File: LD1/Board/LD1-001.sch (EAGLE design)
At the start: 13 parts, among them IC1 TLC5941NT, IC2 TLC5941NT, IC3 TLC5941NT

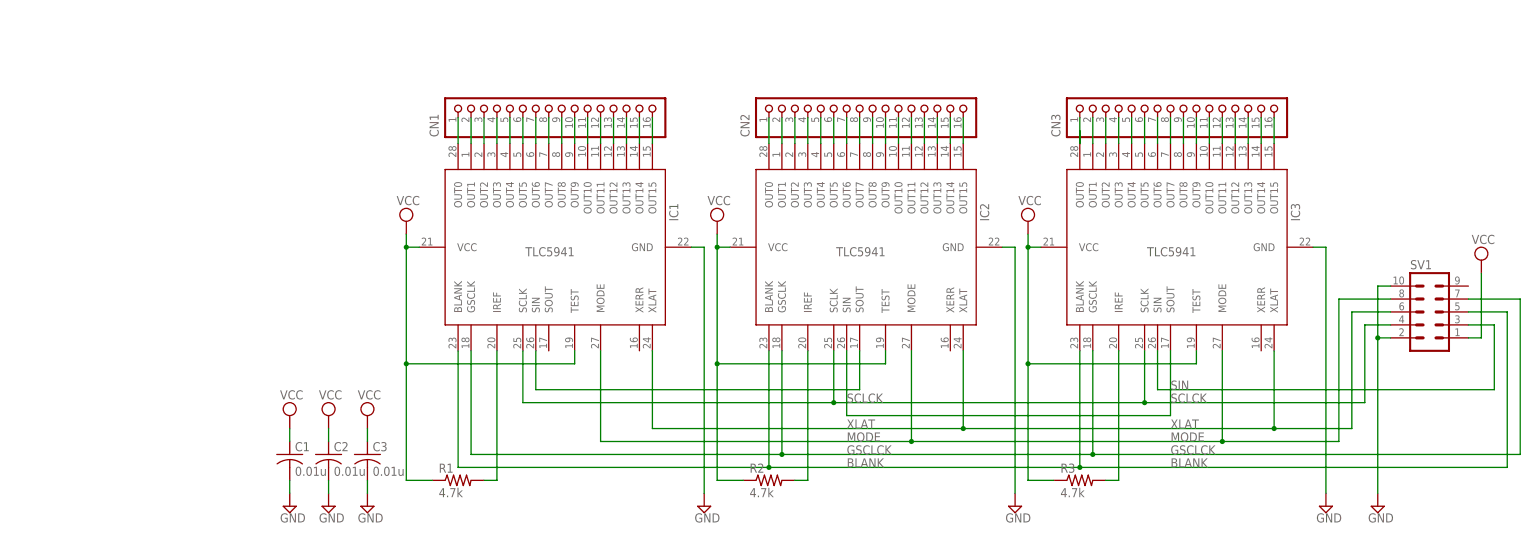
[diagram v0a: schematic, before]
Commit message: Before the first prototyping.
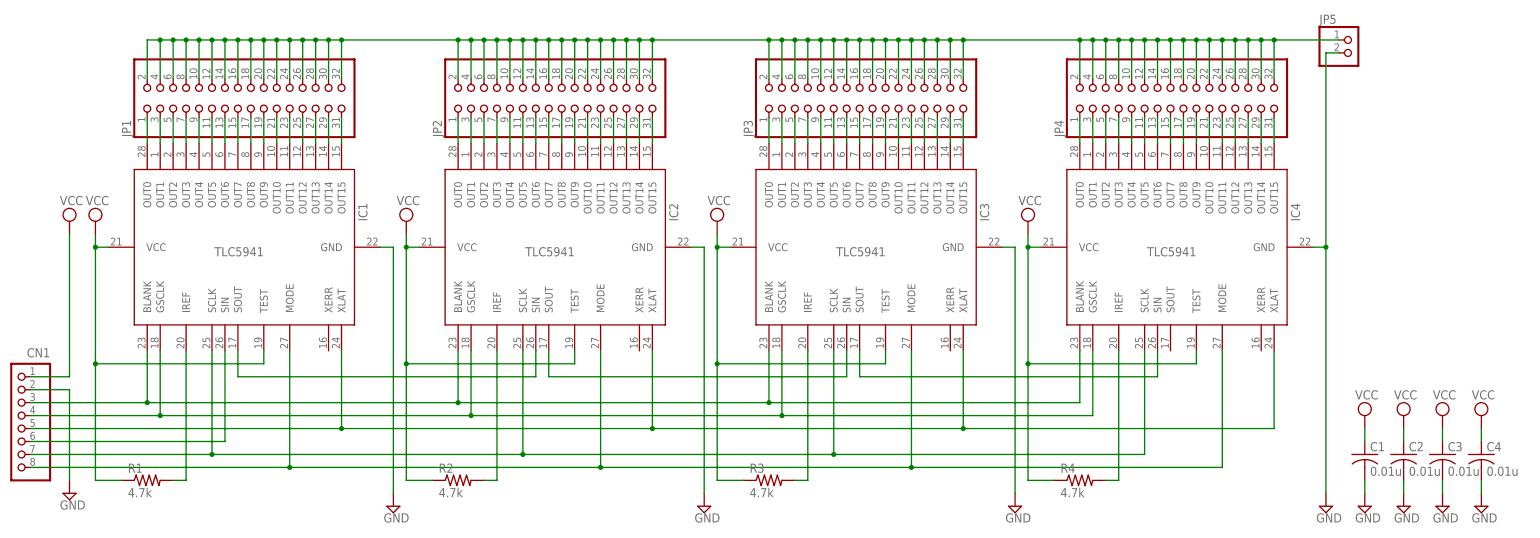
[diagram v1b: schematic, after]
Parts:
- removed CN2, CN3: (no value), jst-ph:B16B-PH-K-S
- removed SV1: (no value), con-ml:ML10
- added C4: 0.01u, rcl:C-US025-025X050
- added IC4: TLC5941NT, adafruit:TLC5941NT
- added JP1, JP2, JP3, JP4: (no value), pinhead:PINHD-2X16
- added JP5: (no value), pinhead:PINHD-1X2
- added R4: 4.7k, resistor:R-US_0204/5
- CN1: device jst-ph:B16B-PH-K-S -> jst-ph:S8B-PH-K-S
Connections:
- removed net LED2B: CN3.6, IC3.OUT5
- removed net LED2G: CN3.5, IC3.OUT4
- removed net LED3B: CN3.9, IC3.OUT8
- removed net LED3G: CN3.8, IC3.OUT7
- removed net LED3R: CN3.7, IC3.OUT6
- removed net LEDA: CN3.1, IC3.OUT0
- removed net SIN: IC3.SIN, SV1.3
- new net N$37: IC4.IREF, R4.2
- new net N$48: IC3.OUT8, JP3.17
- new net N$49: IC3.OUT9, JP3.19
- new net N$50: IC3.OUT10, JP3.21
- new net N$51: IC3.OUT11, JP3.23
- new net N$52: IC3.OUT12, JP3.25
- new net N$53: IC3.OUT13, JP3.27
- new net N$54: IC3.OUT14, JP3.29
- new net N$55: IC3.OUT15, JP3.31
- new net N$56: IC4.OUT0, JP4.1
- new net N$57: IC4.OUT1, JP4.3
- new net N$58: IC4.OUT2, JP4.5
- new net N$59: IC4.OUT3, JP4.7
- new net N$60: IC4.OUT4, JP4.9
- new net N$61: IC4.OUT5, JP4.11
- new net N$62: IC4.OUT6, JP4.13
- new net N$63: IC4.OUT7, JP4.15
- new net N$64: IC4.OUT8, JP4.17
- new net N$66: IC4.OUT9, JP4.19
- new net N$67: IC4.OUT10, JP4.21
- new net N$68: IC4.OUT11, JP4.23
- new net N$69: IC4.OUT12, JP4.25
- new net N$70: IC4.OUT13, JP4.27
- new net N$71: IC4.OUT14, JP4.29
- new net N$72: IC4.OUT15, JP4.31
- new net N$73: JP1.10, JP1.12, JP1.14, JP1.16, JP1.18, JP1.2, JP1.20, JP1.22, JP1.24, JP1.26, JP1.28, JP1.30, JP1.32, JP1.4, JP1.6, JP1.8, JP2.10, JP2.12, JP2.14, JP2.16, JP2.18, JP2.2, JP2.20, JP2.22, JP2.24, JP2.26, JP2.28, JP2.30, JP2.32, JP2.4, JP2.6, JP2.8, JP3.10, JP3.12, JP3.14, JP3.16, JP3.18, JP3.2, JP3.20, JP3.22, JP3.24, JP3.26, JP3.28, JP3.30, JP3.32, JP3.4, JP3.6, JP3.8, JP4.10, JP4.12, JP4.14, JP4.16, JP4.18, JP4.2, JP4.20, JP4.22, JP4.24, JP4.26, JP4.28, JP4.30, JP4.32, JP4.4, JP4.6, JP4.8, JP5.1
- net BLANK: now also CN1.3, IC4.BLANK; no longer SV1.5
- net GND: now also C4.2, CN1.2, IC4.GND, JP5.2; no longer SV1.10, SV1.2
- net GSCLCK: now also CN1.4, IC4.GSCLK; no longer SV1.7
- net MODE: now also CN1.8, IC4.MODE; no longer SV1.8
- net N$1: now also CN1.6, IC1.SIN; no longer CN2.16, IC2.OUT15
- net N$10: now also IC1.OUT5, JP1.11; no longer IC2.SIN, IC3.SOUT
- net N$11: now also IC1.OUT6, JP1.13; no longer CN2.4, IC2.OUT3
- net N$12: now also IC1.OUT7, JP1.15; no longer CN3.2, IC3.OUT1
- net N$13: now also IC1.OUT8, JP1.17; no longer CN2.5, IC2.OUT4
- net N$14: now also IC1.OUT9, JP1.19; no longer CN3.3, IC3.OUT2
- net N$15: now also IC1.OUT10, JP1.21; no longer CN2.6, IC2.OUT5
- net N$16: now also IC1.OUT11, JP1.23; no longer CN2.7, IC2.OUT6
- net N$17: now also IC1.OUT12, JP1.25; no longer CN2.8, IC2.OUT7
- net N$18: now also IC1.OUT13, JP1.27; no longer CN2.9, IC2.OUT8
- net N$19: now also IC1.OUT14, JP1.29; no longer CN2.10, IC2.OUT9
- net N$2: now also IC1.SOUT, IC2.SIN; no longer CN2.2, IC2.OUT1
- net N$20: now also IC1.OUT15, JP1.31; no longer CN2.11, IC2.OUT10
- net N$21: now also IC2.OUT0, JP2.1; no longer CN2.12, IC2.OUT11
- net N$22: now also IC2.OUT1, JP2.3; no longer CN2.13, IC2.OUT12
- net N$23: now also IC2.OUT2, JP2.5; no longer CN2.14, IC2.OUT13
- net N$24: now also IC2.OUT3, JP2.7; no longer CN3.15, IC3.OUT14
- net N$25: now also IC2.OUT4, JP2.9; no longer CN3.16, IC3.OUT15
- net N$26: now also IC2.OUT5, JP2.11; no longer CN2.15, IC2.OUT14
- net N$27: now also IC2.OUT6, JP2.13; no longer CN2.1, IC2.OUT0
- net N$28: now also IC2.OUT7, JP2.15; no longer CN1.16, IC1.OUT15
- net N$29: now also IC2.OUT8, JP2.17; no longer CN1.15, IC1.OUT14
- net N$3: now also IC2.SOUT, IC3.SIN; no longer CN3.13, IC3.OUT12
- net N$30: now also IC2.OUT9, JP2.19; no longer CN1.14, IC1.OUT13
- net N$31: now also IC2.OUT10, JP2.21; no longer CN1.13, IC1.OUT12
- net N$32: now also IC2.OUT11, JP2.23; no longer CN1.12, IC1.OUT11
- net N$33: now also IC2.OUT12, JP2.25; no longer CN1.11, IC1.OUT10
- net N$34: now also IC2.OUT13, JP2.27; no longer CN1.10, IC1.OUT9
- net N$35: now also IC2.OUT14, JP2.29; no longer CN1.9, IC1.OUT8
- net N$36: now also IC2.OUT15, JP2.31; no longer CN1.8, IC1.OUT7
- net N$38: now also IC3.OUT0, JP3.1; no longer CN1.7, IC1.OUT6
- net N$39: now also IC3.OUT1, JP3.3; no longer CN1.6, IC1.OUT5
- net N$4: now also IC3.SOUT, IC4.SIN; no longer CN2.3, IC2.OUT2
- net N$40: now also IC3.OUT2, JP3.5; no longer CN1.5, IC1.OUT4
- net N$41: now also IC3.OUT3, JP3.7; no longer CN1.4, IC1.OUT3
- net N$42: now also IC3.OUT4, JP3.9; no longer CN1.3, IC1.OUT2
- net N$43: now also IC3.OUT5, JP3.11; no longer CN1.2, IC1.OUT1
- net N$44: now also IC3.OUT6, JP3.13; no longer CN1.1, IC1.OUT0
- net N$45: now also IC3.OUT7, JP3.15; no longer IC1.SIN, IC2.SOUT
- net N$5: now also IC1.OUT0, JP1.1; no longer CN3.14, IC3.OUT13
- net N$6: now also IC1.OUT1, JP1.3; no longer CN3.10, IC3.OUT9
- net N$7: now also IC1.OUT2, JP1.5; no longer CN3.11, IC3.OUT10
- net N$8: now also IC1.OUT3, JP1.7; no longer CN3.12, IC3.OUT11
- net N$9: now also IC1.OUT4, JP1.9; no longer CN3.4, IC3.OUT3
- net SCLCK: now also CN1.7, IC4.SCLK; no longer SV1.4
- net VCC: now also C4.1, CN1.1, IC4.TEST, IC4.VCC, R4.1; no longer SV1.1
- net XLAT: now also CN1.5, IC4.XLAT; no longer SV1.6
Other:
- moved on the sheet: C1, C2, C3, IC1, IC2, IC3, R1, R2, R3
